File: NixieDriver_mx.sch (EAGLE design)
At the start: 18 parts, among them IC1 PIC18F2550_28DIP, IC2 74141N, Q1 20MHz, T1 BF420, T2 BF420, T3 BF420, X1 USB-B-H

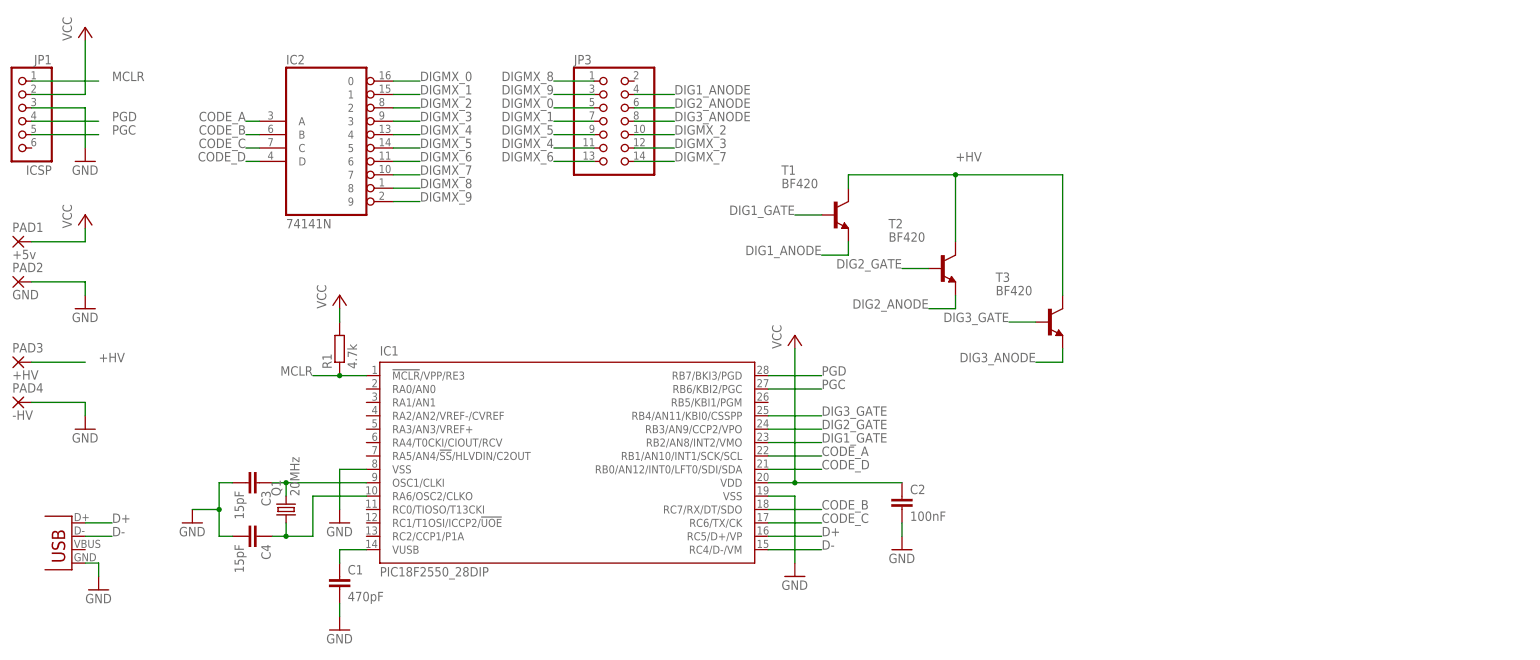
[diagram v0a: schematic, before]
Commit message: Dump current status from laptop
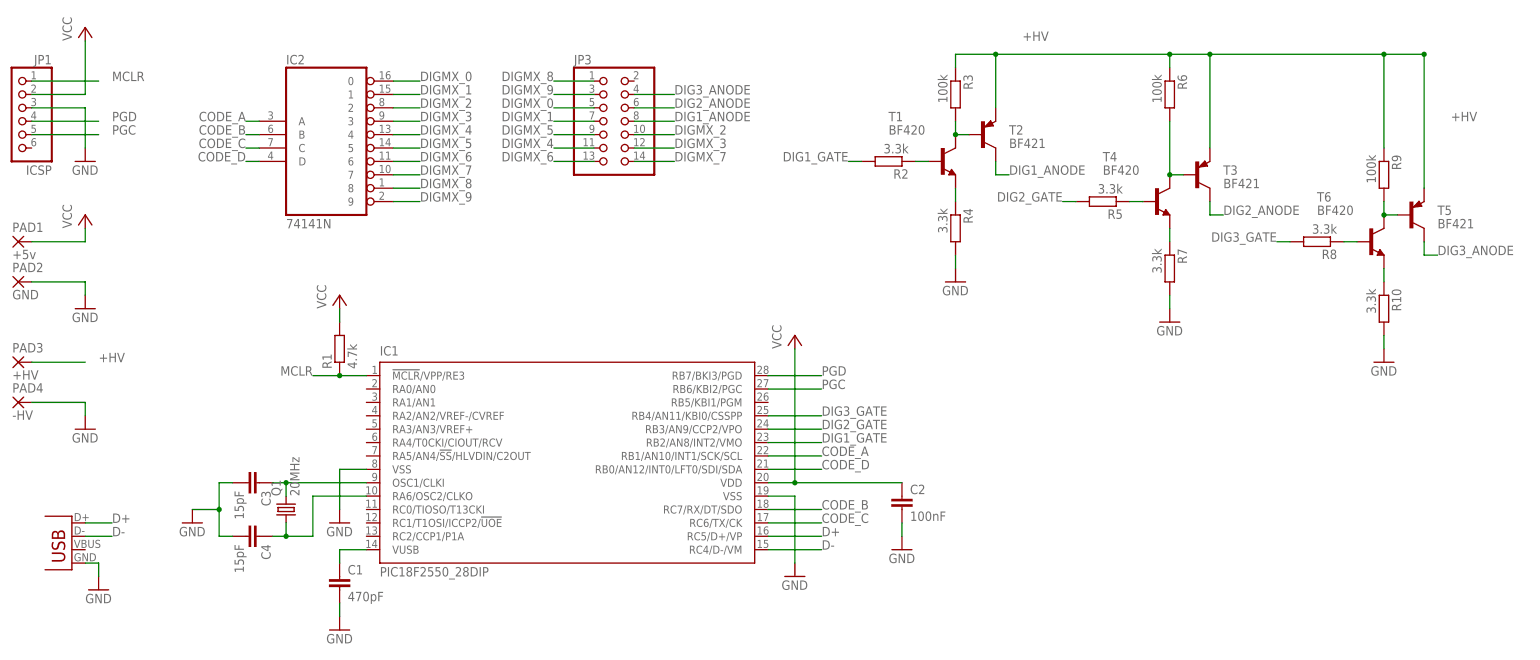
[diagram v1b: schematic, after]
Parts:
- added R10, R4, R7: 3.3k, rcl:R-EU_0207/7
- added R2, R5, R8: 3.3k, rcl:R-EU_0207/2V
- added R3, R6, R9: 100k, rcl:R-EU_0207/5V
- added T4, T6: BF420, transistor-neu-to92:BC368-NPN-TO92-ECB
- added T5: BF421, transistor-neu-to92:-PNP-TO92-ECB
- T1: device transistor:BF420-NPN-TO92-BCE -> transistor-neu-to92:BC368-NPN-TO92-ECB
- T2, T3: value BF420 -> BF421; device transistor:BF420-NPN-TO92-BCE -> transistor-neu-to92:-PNP-TO92-ECB
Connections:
- new net N$10: R9.2, T5.B, T6.C
- new net N$11: R10.1, T6.E
- new net N$12: R8.1, T6.B
- new net N$4: R3.2, T1.C, T2.B
- new net N$5: R2.1, T1.B
- new net N$6: R4.1, T1.E
- new net N$7: R6.2, T3.B, T4.C
- new net N$8: R7.1, T4.E
- new net N$9: R5.1, T4.B
- net +HV: now also R3.1, R6.1, R9.1, T2.E, T3.E, T5.E; no longer T1.C, T2.C, T3.C
- net DIG1_ANODE: now also JP3.8, T2.C; no longer JP3.4, T1.E
- net DIG1_GATE: now also R2.2; no longer T1.B
- net DIG2_ANODE: now also T3.C; no longer T2.E
- net DIG2_GATE: now also R5.2; no longer T2.B
- net DIG3_ANODE: now also JP3.4, T5.C; no longer JP3.8, T3.E
- net DIG3_GATE: now also R8.2; no longer T3.B
- net GND: now also R10.2, R4.2, R7.2
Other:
- moved on the sheet: T1
